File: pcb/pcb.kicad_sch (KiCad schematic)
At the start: 6 parts, among them J1 Connector, USB-TYPE-C-16P, U1 MCP1700x-330xxTT

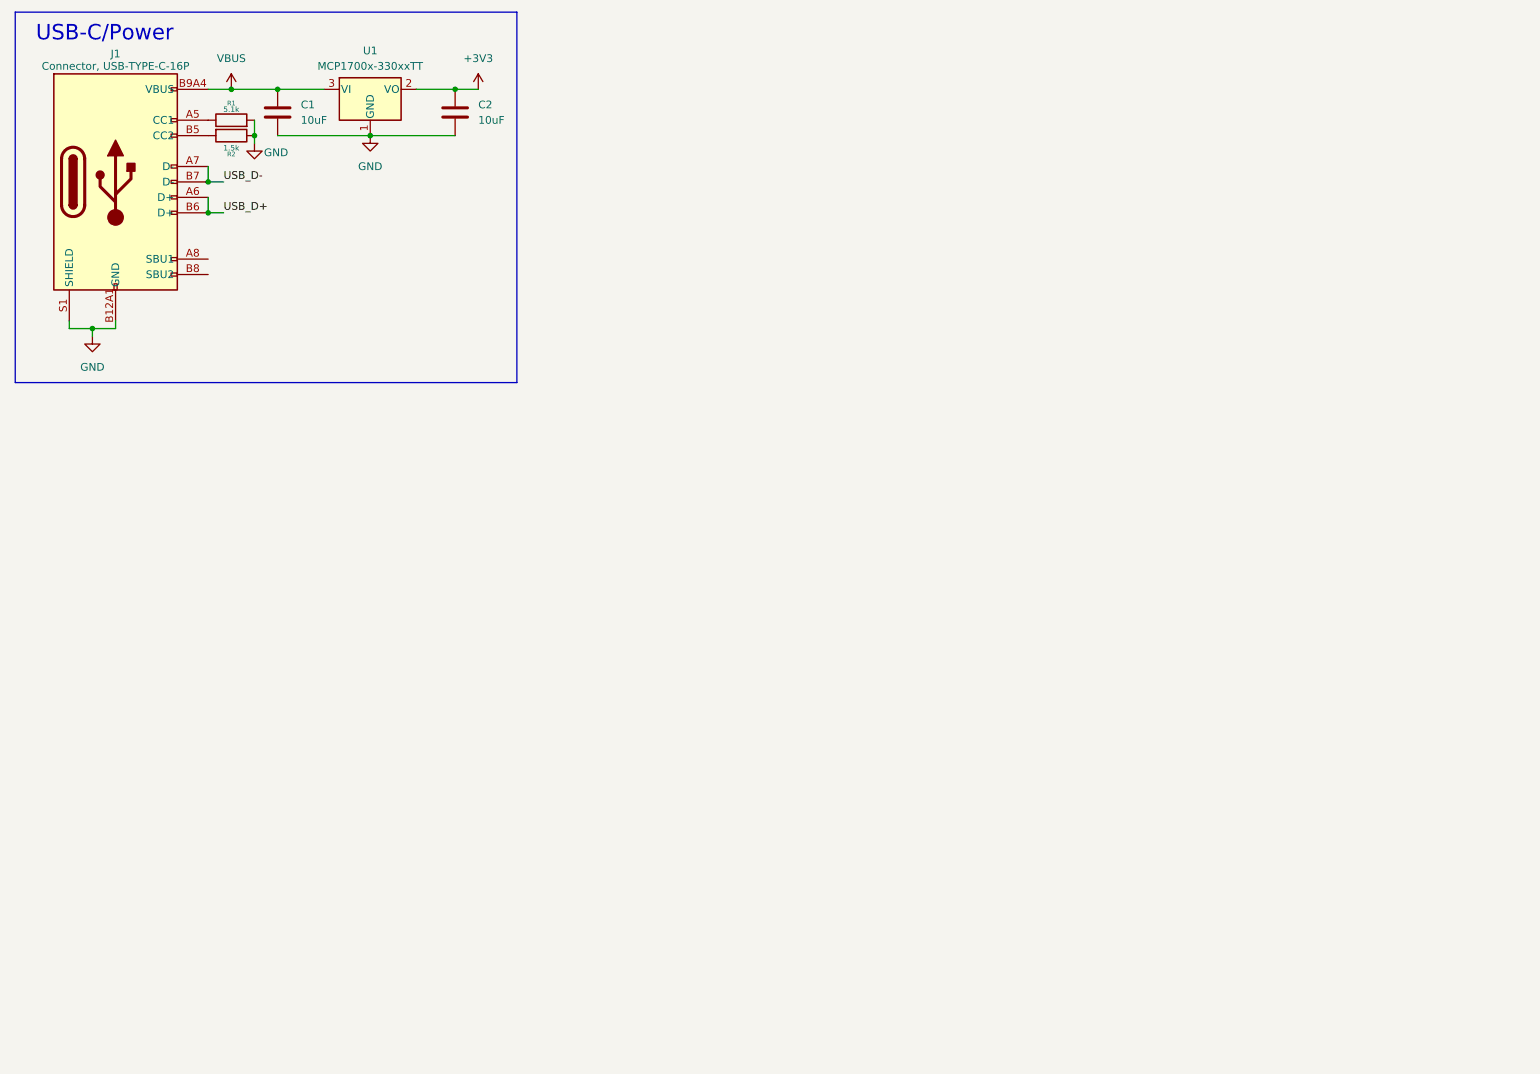
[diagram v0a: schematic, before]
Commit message: more pcb work
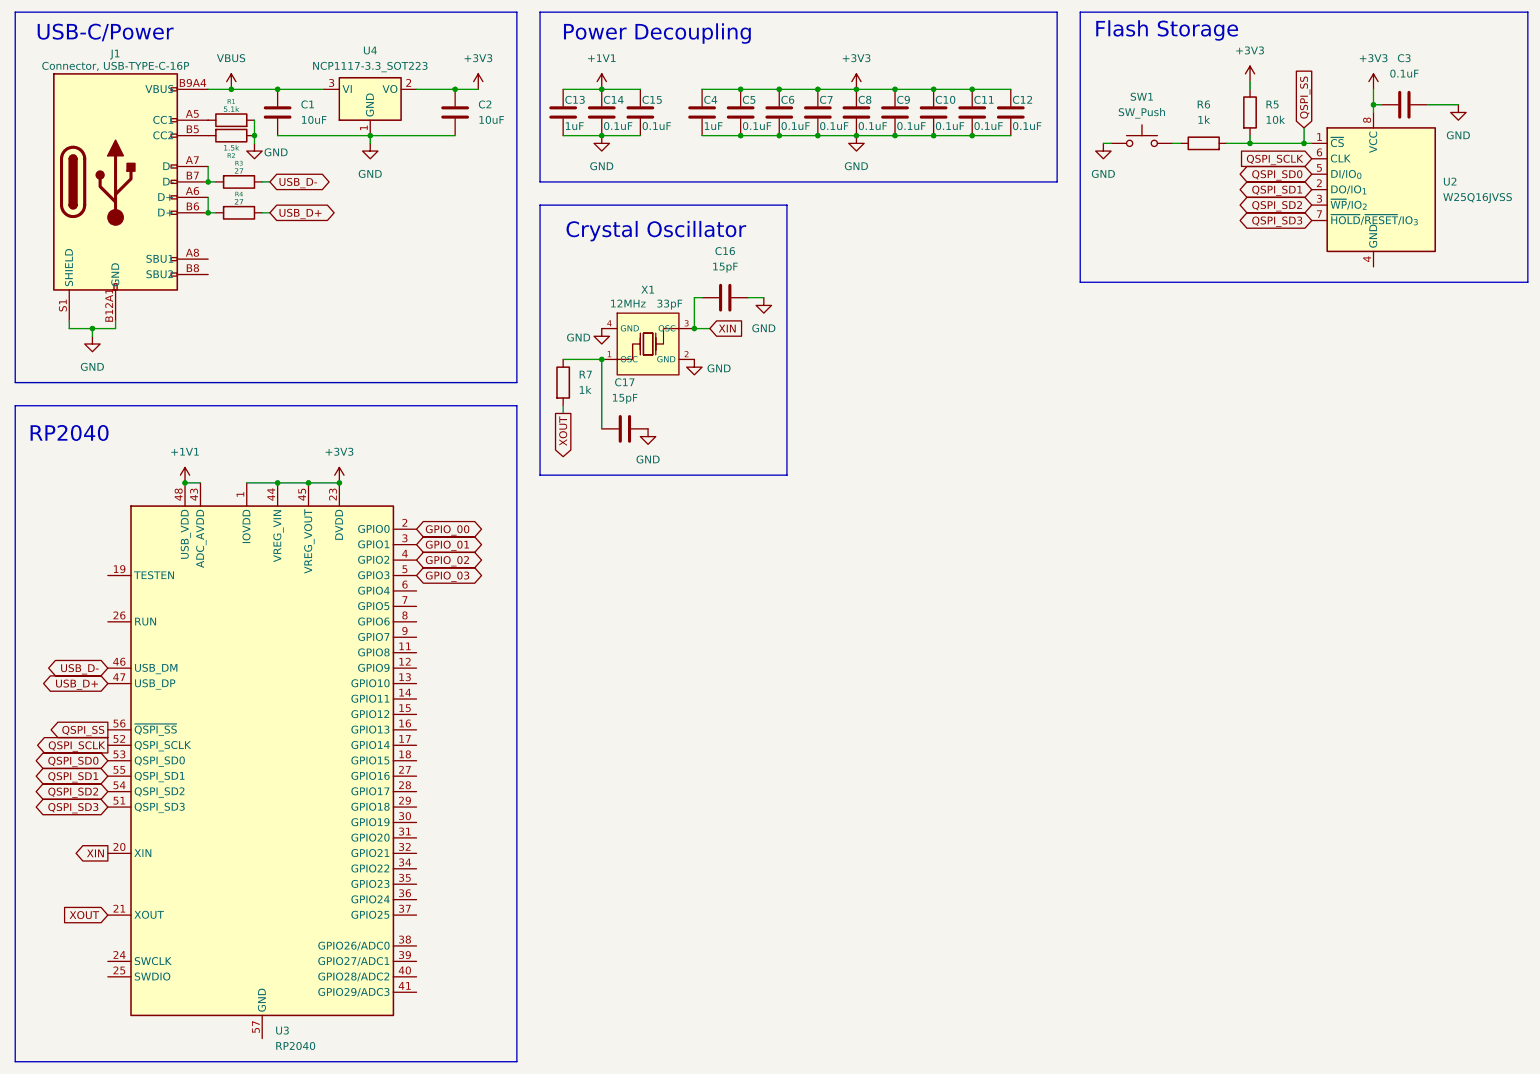
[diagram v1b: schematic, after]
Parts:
- removed U1: MCP1700x-330xxTT, Package_TO_SOT_SMD:SOT-23, symbol Regulator_Linear:MCP1700x-330xxTT
- added C10, C11, C12, C14, C15, C3, C5, C6, C7, C8, C9: 0.1uF, Capacitor_SMD:C_0805_2012Metric, symbol Device:C
- added C13, C4: 1uF, Capacitor_SMD:C_0805_2012Metric, symbol Device:C
- added C16, C17: 15pF, Capacitor_SMD:C_0805_2012Metric, symbol Device:C
- added R3, R4: 27, Resistor_SMD:R_0603_1608Metric, symbol Device:R
- added R5: 10k, Resistor_SMD:R_0603_1608Metric, symbol Device:R
- added R6, R7: 1k, Resistor_SMD:R_0603_1608Metric, symbol Device:R
- added SW1: SW_Push, symbol Switch:SW_Push
- added U2: W25Q16JVSS, Package_SO:SOIC-8_5.3x5.3mm_P1.27mm, symbol Memory_Flash:W25Q16JVSS
- added U3: RP2040, Package_DFN_QFN:QFN-56-1EP_7x7mm_P0.4mm_EP3.2x3.2mm, symbol MCU_RaspberryPi:RP2040
- added U4: NCP1117-3.3_SOT223, Package_TO_SOT_SMD:SOT-223-3_TabPin2, symbol Regulator_Linear:NCP1117-3.3_SOT223
- added X1: X322512MSB4SI, PCM_JLCPCB:CRYSTAL-SMD_4P-L3.2-W2.5-BL, symbol PCM_JLCPCB-Crystals:Crystal, 12MHz, 20pF
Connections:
- net +3V3: now also C10.1, C11.1, C12.1, C3.1, C4.1, C5.1, C6.1, C7.1, C8.1, C9.1, R5.1, U2.8 (VCC), U3.1 (IOVDD), U3.10 (IOVDD), U3.22 (IOVDD), U3.23 (DVDD), U3.33 (IOVDD), U3.42 (IOVDD), U3.44 (VREG_VIN), U3.45 (VREG_VOUT), U3.49 (IOVDD), U3.50 (DVDD), U4.2 (VO)
- net GND: now also C10.2, C11.2, C12.2, C13.2, C14.2, C15.2, C16.1, C17.1, C3.2, C4.2, C5.2, C6.2, C7.2, C8.2, C9.2, SW1.1, U4.1 (GND), X1.2 (GND), X1.4 (GND)
- net USB_D+: now also R4.1, U3.47 (USB_DP); no longer J1.A6 (D+), J1.B6 (D+)
- net USB_D-: now also R3.1, U3.46 (USB_DM); no longer J1.A7 (D-), J1.B7 (D-)
- net VBUS: now also U4.3 (VI)
- new net: J1.A6 (D+), J1.B6 (D+), R4.2
- new net: J1.A7 (D-), J1.B7 (D-), R3.2
- new net: C17.2, R7.1, X1.1 (OSC)
- new net: R6.1, SW1.2
- new net +1V1: C13.1, C14.1, C15.1, U3.43 (ADC_AVDD), U3.48 (USB_VDD)
- new net GPIO_00: U3.2 (GPIO0)
- new net GPIO_01: U3.3 (GPIO1)
- new net GPIO_02: U3.4 (GPIO2)
- new net GPIO_03: U3.5 (GPIO3)
- new net QSPI_SCLK: U2.6 (CLK), U3.52 (QSPI_SCLK)
- new net QSPI_SD0: U2.5 (DI/IO_{0}), U3.53 (QSPI_SD0)
- new net QSPI_SD1: U2.2 (DO/IO_{1}), U3.55 (QSPI_SD1)
- new net QSPI_SD2: U2.3 (~{WP}/IO_{2}), U3.54 (QSPI_SD2)
- new net QSPI_SD3: U2.7 (~{HOLD}/~{RESET}/IO_{3}), U3.51 (QSPI_SD3)
- new net QSPI_SS: R5.2, R6.2, U2.1 (~{CS}), U3.56 (~{QSPI_SS})
- new net XIN: C16.2, U3.20 (XIN), X1.3 (OSC)
- new net XOUT: R7.2, U3.21 (XOUT)
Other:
- note added: "Crystal Oscillator"
- note added: "Flash Storage"
- note added: "Power Decoupling"
- note added: "RP2040"
